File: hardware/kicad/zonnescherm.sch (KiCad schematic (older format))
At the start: 26 parts, among them K1 K1-ON/OFF, K2 K1-UP/DOWN, K3 K2-ON/OFF, K4 K2-UP/DOWN, P1 ARDUINO-ISP, P2 CONN_MAINS, P3 CONN_SUNSHADE1, P4 CONN_SUNSHADE2, P5 CONN_02X04, U1 IRM-05-5, U2 LM1117-3.3, U3 ESP-12E, U4 ULN2003A

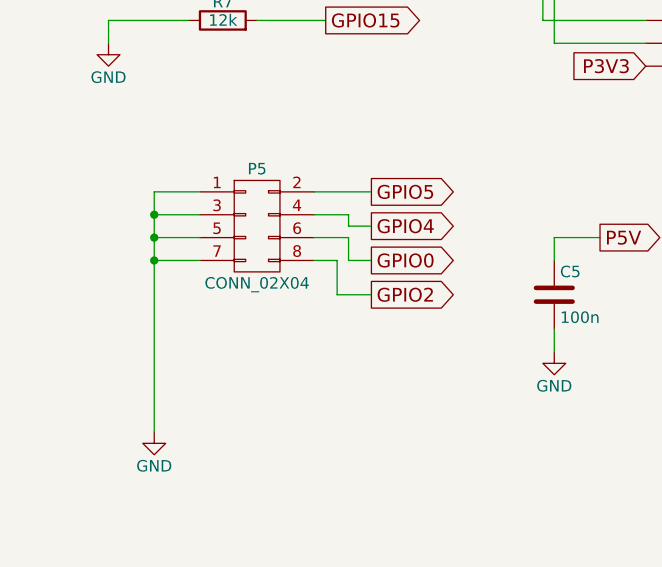
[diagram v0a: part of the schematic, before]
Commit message: Added logo
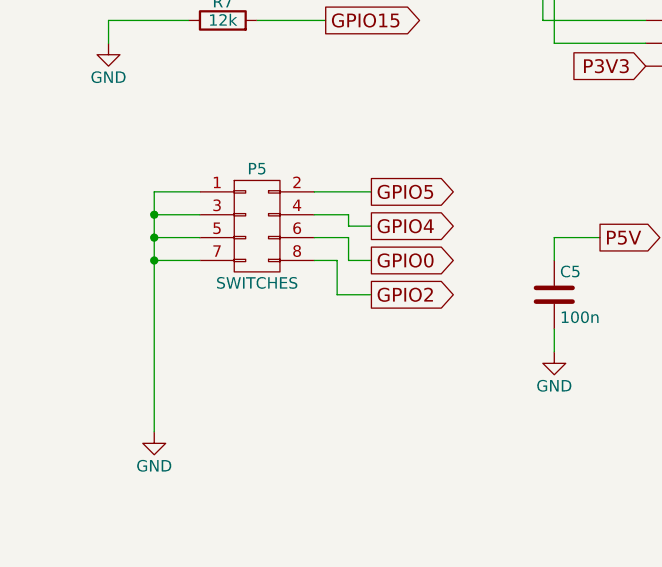
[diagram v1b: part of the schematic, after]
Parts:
- P5: value CONN_02X04 -> SWITCHES
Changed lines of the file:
@@
 P 1800 4900
 F 0 "P5" H 1800 5150 50  0000 C CNN
-F 1 "CONN_02X04" H 1800 4650 50  0000 C CNN
+F 1 "SWITCHES" H 1800 4650 50  0000 C CNN
 F 2 "Pin_Headers:Pin_Header_Straight_2x04" H 1800 3700 50  0001 C CNN
 F 3 "" H 1800 3700 50  0000 C CNN

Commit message: Updated layout, added text etc.
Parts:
- C1: footprint Capacitors_SMD:c_elec_5x5.3 -> Capacitors_SMD:c_elec_8x6.5
- C4: footprint Capacitors_SMD:c_elec_5x5.3 -> Capacitors_SMD:c_elec_4x5.8
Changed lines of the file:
@@
 F 0 "C4" H 5025 1950 50  0000 L CNN
 F 1 "10u/16V" H 5025 1750 50  0000 L CNN
-F 2 "Capacitors_SMD:c_elec_5x5.3" H 5038 1700 50  0001 C CNN
+F 2 "Capacitors_SMD:c_elec_4x5.8" H 5038 1700 50  0001 C CNN
 F 3 "" H 5000 1850 50  0000 C CNN
 	1    5000 1850
@@
 F 0 "C1" H 3575 1950 50  0000 L CNN
 F 1 "100u/16V" H 3575 1750 50  0000 L CNN
-F 2 "Capacitors_SMD:c_elec_5x5.3" H 3588 1700 50  0001 C CNN
+F 2 "Capacitors_SMD:c_elec_8x6.5" H 3588 1700 50  0001 C CNN
 F 3 "" H 3550 1850 50  0000 C CNN
 	1    3550 1850
